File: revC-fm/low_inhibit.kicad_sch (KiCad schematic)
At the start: 14 parts, among them Q2 MMDT2907AQ, Q55 MMDT3946, Q56 BSZ025N04LSATMA1, Q57 BSZ025N04LSATMA1

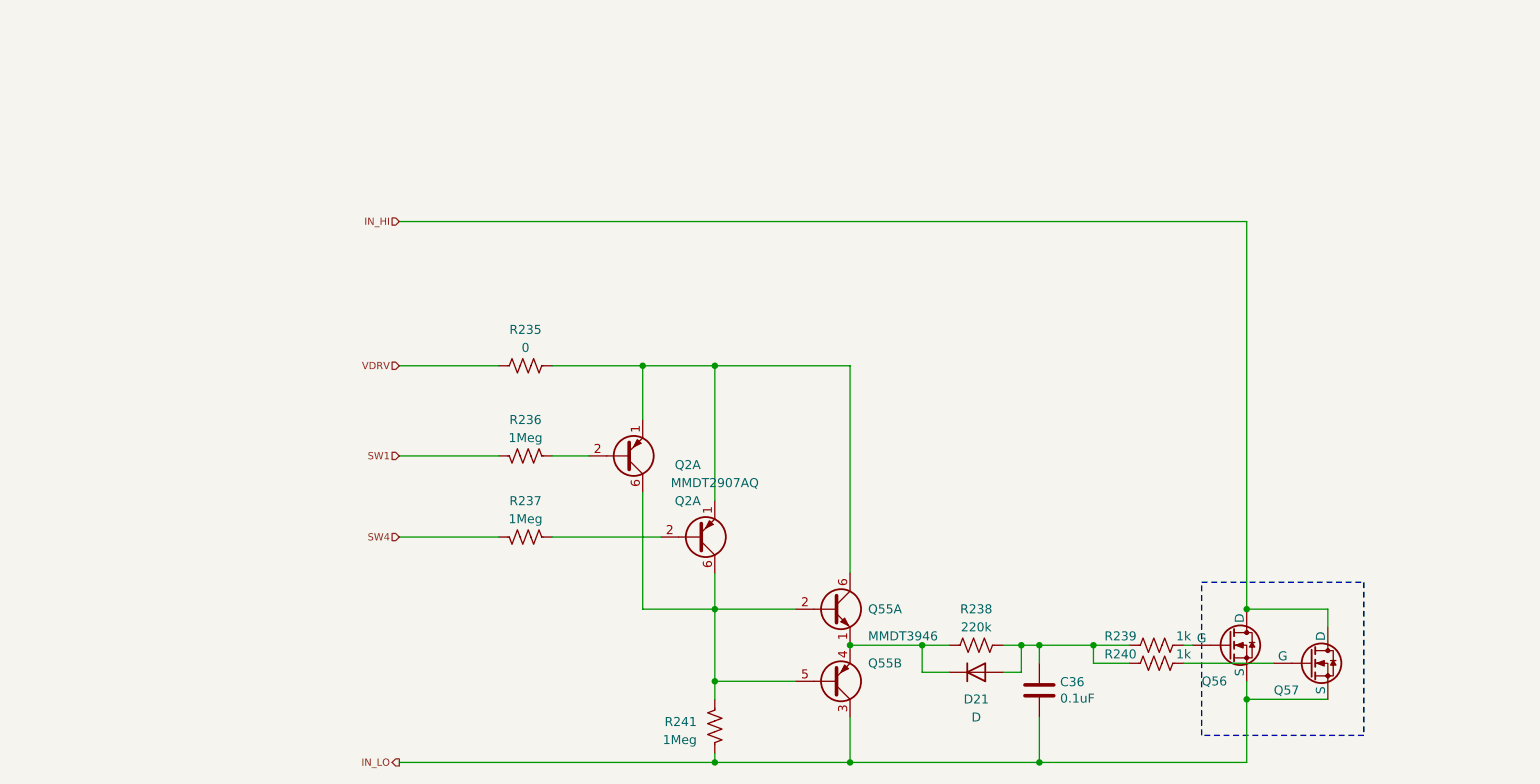
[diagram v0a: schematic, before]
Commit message: almost done!!!!!
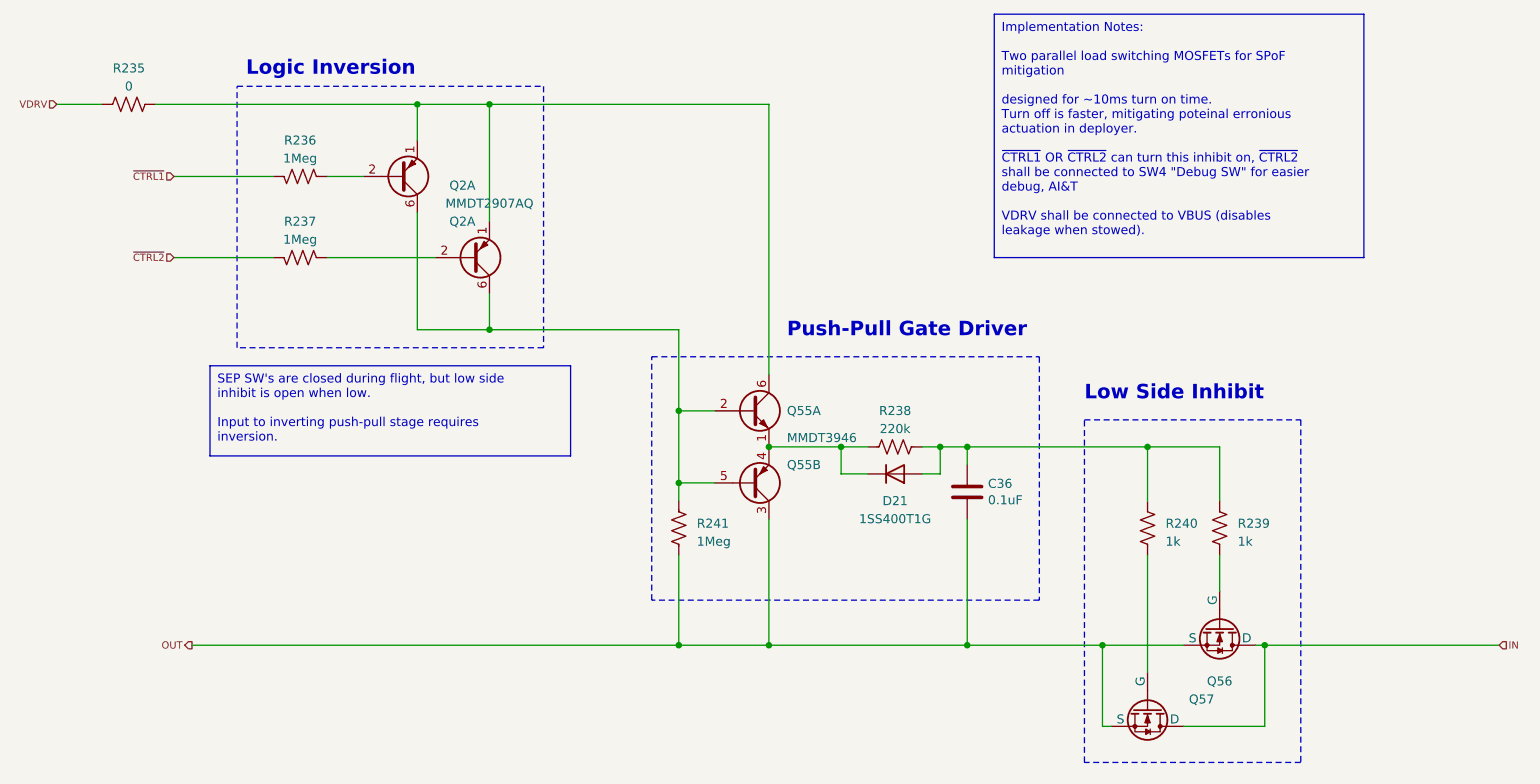
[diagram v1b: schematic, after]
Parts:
- D21: value D -> 1SS400T1G
- Q56, Q57: value BSZ025N04LSATMA1 -> BSZ025; Mfr. Part No BSZ025N04LS -> BSZ025N04LSATMA1
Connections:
- net at C36.1, D21.2 (A), R238.2: now also R239.2, R240.2; no longer R239.1, R240.1
- net at Q56.4 (G): now also R239.1; no longer R239.2
- net at Q57.4 (G): now also R240.1; no longer R240.2
- net IN_HI renamed IN
- net IN_LO renamed OUT
- net SW1 renamed ~{CTRL1}
- net SW4 renamed ~{CTRL2}
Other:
- note added: "Logic Inversion"
- note added: "Low Side Inhibit"
- note added: "Push-Pull Gate Driver"
- moved on the sheet: C36, D21, Q2A, Q55A, Q55B, Q56, Q57, R235, R236, R237, R238, R239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
